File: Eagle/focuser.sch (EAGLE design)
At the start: 14 parts, among them IC1 L293D, IC2 L293D, IC3 PCF8574P

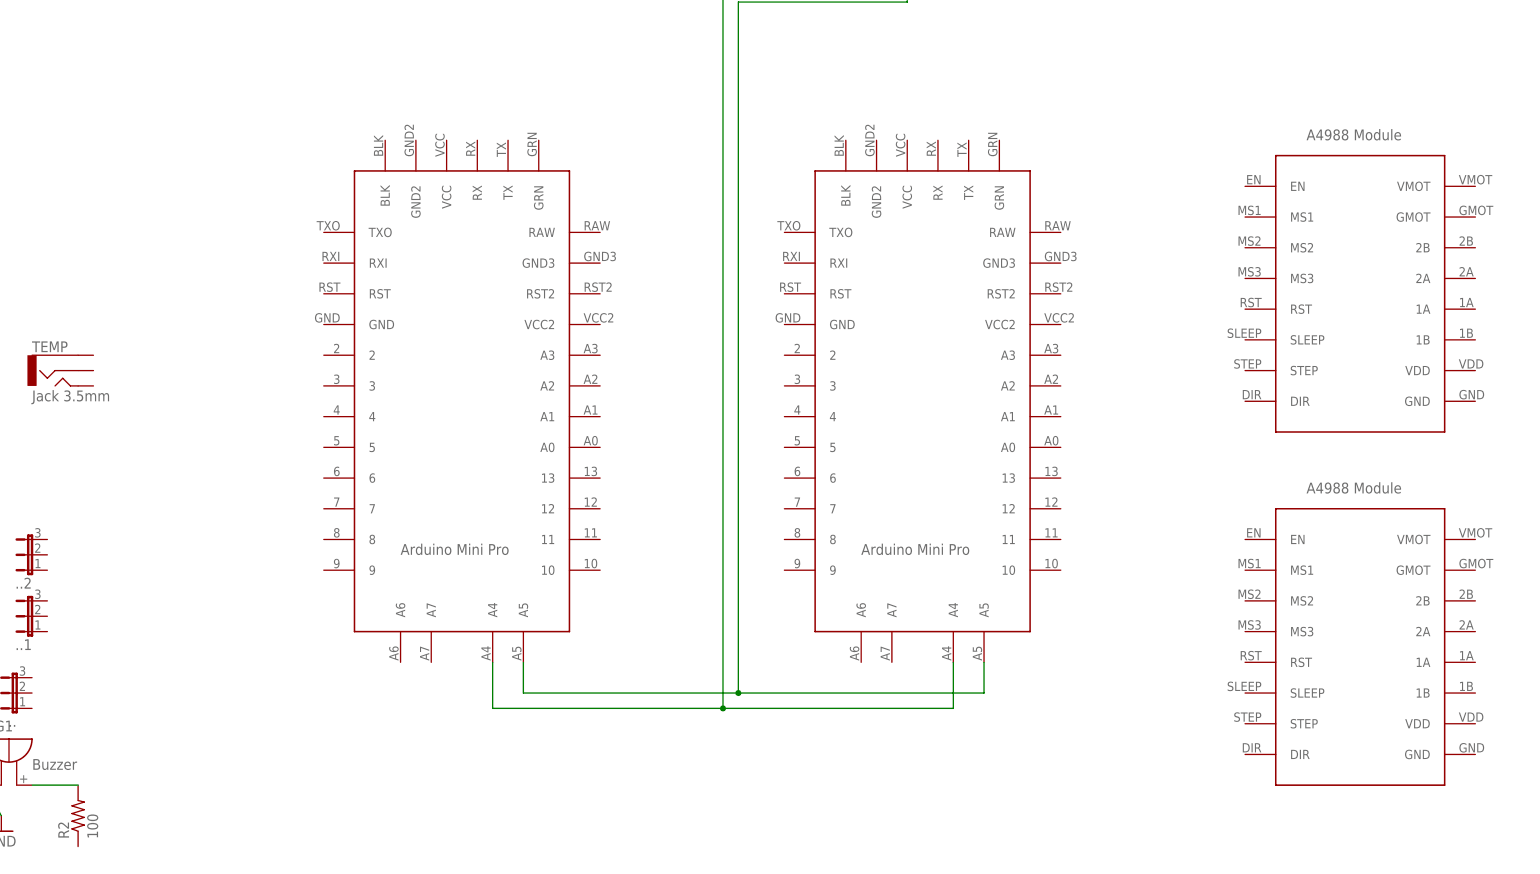
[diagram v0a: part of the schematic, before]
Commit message: Work continues... VB script update
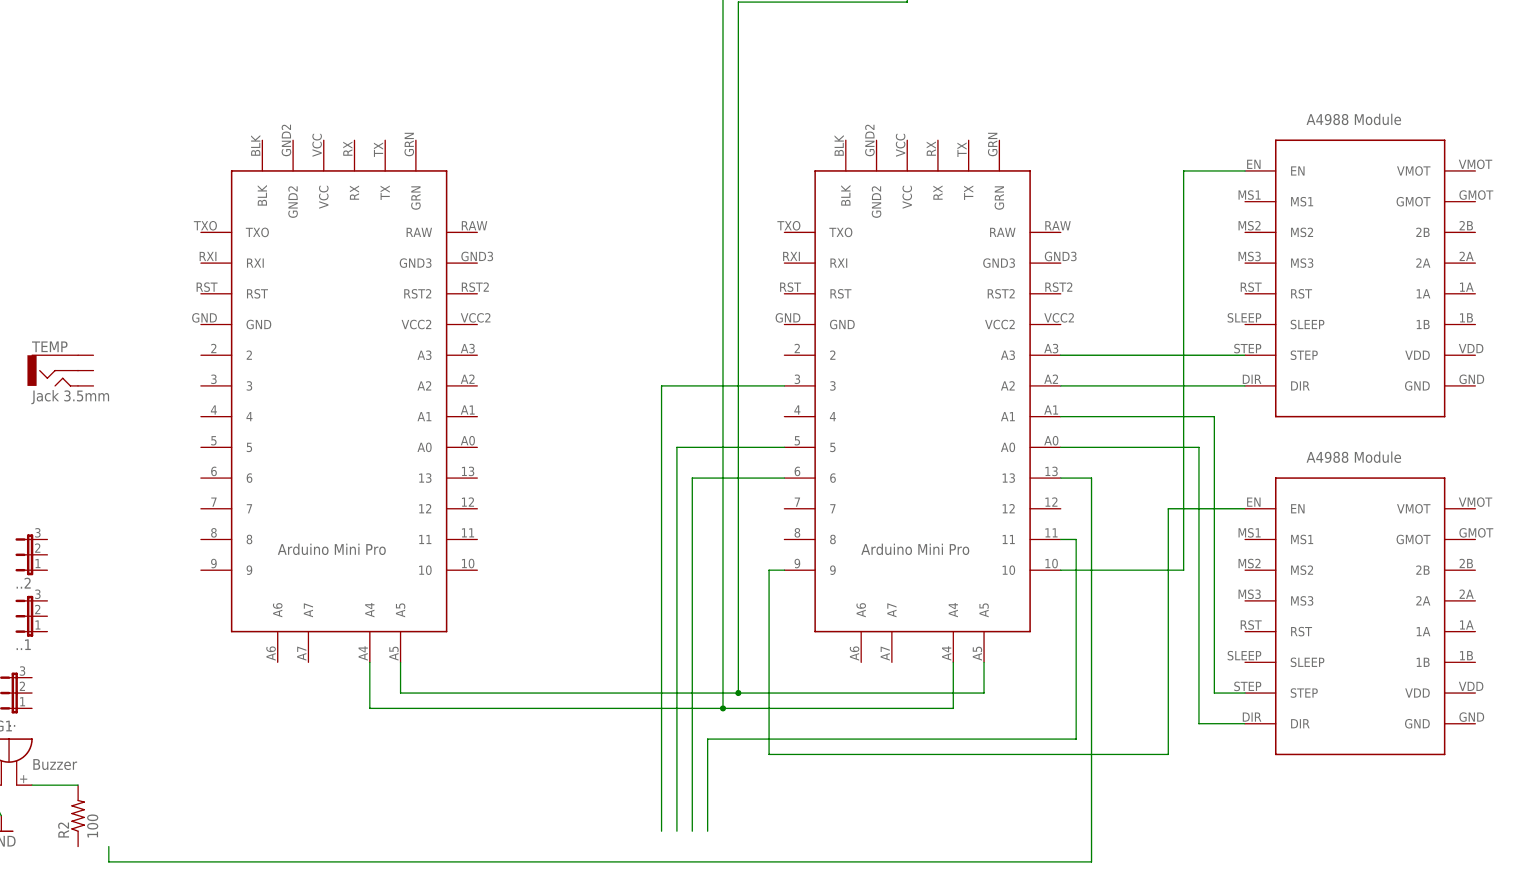
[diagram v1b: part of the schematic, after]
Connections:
- new net N$10: U$1.6
- new net N$11: U$1.5
- new net N$12: U$1.3
- new net N$13: U$1.11
- new net N$14: U$1.13
- new net N$3: U$1.A3, U$7.STEP
- new net N$4: U$1.A2, U$7.DIR
- new net N$5: U$1.A1, U$6.STEP
- new net N$6: U$1.A0, U$6.DIR
- new net N$7: U$1.10, U$7.EN
- new net N$8: U$1.9, U$6.EN
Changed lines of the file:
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@@
 <instance part="..2" gate="G$1" x="-33.02" y="45.72" rot="R90"/>
 <instance part="U$1" gate="G$1" x="116.84" y="81.28"/>
-<instance part="U$6" gate="G$1" x="182.88" y="38.1"/>
-<instance part="U$7" gate="G$1" x="182.88" y="96.52"/>
-<instance part="U$8" gate="G$1" x="40.64" y="81.28"/>
+<instance part="U$6" gate="G$1" x="182.88" y="43.18"/>
+<instance part="U$7" gate="G$1" x="182.88" y="99.06"/>
+<instance part="U$8" gate="G$1" x="20.32" y="81.28"/>
 <instance part="IC1" gate="G$1" x="190.5" y="160.02" rot="R90"/>
 <instance part="IC2" gate="G$1" x="190.5" y="210.82" rot="R90"/>
@@
 <net name="N$1" class="0">
 <segment>
-<pinref part="U$8" gate="G$1" pin="A5"/>
-<wire x1="48.26" y1="30.48" x2="48.26" y2="25.4" width="0.1524" layer="91"/>
-<wire x1="48.26" y1="25.4" x2="83.82" y2="25.4" width="0.1524" layer="91"/>
+<wire x1="27.94" y1="25.4" x2="83.82" y2="25.4" width="0.1524" layer="91"/>
 <pinref part="U$1" gate="G$1" pin="A5"/>
 <wire x1="83.82" y1="25.4" x2="124.46" y2="25.4" width="0.1524" layer="91"/>
@@
 <wire x1="83.82" y1="139.7" x2="83.82" y2="25.4" width="0.1524" layer="91"/>
 <junction x="83.82" y="25.4"/>
+<pinref part="U$8" gate="G$1" pin="A5"/>
+<wire x1="27.94" y1="30.48" x2="27.94" y2="25.4" width="0.1524" layer="91"/>
 </segment>
 </net>
 <net name="N$2" class="0">
 <segment>
-<pinref part="U$8" gate="G$1" pin="A4"/>
-<wire x1="43.18" y1="30.48" x2="43.18" y2="22.86" width="0.1524" layer="91"/>
-<wire x1="43.18" y1="22.86" x2="81.28" y2="22.86" width="0.1524" layer="91"/>
+<wire x1="22.86" y1="22.86" x2="81.28" y2="22.86" width="0.1524" layer="91"/>
 <pinref part="U$1" gate="G$1" pin="A4"/>
 <wire x1="81.28" y1="22.86" x2="119.38" y2="22.86" width="0.1524" layer="91"/>
@@
 <wire x1="81.28" y1="142.24" x2="81.28" y2="22.86" width="0.1524" layer="91"/>
 <junction x="81.28" y="22.86"/>
+<pinref part="U$8" gate="G$1" pin="A4"/>
+<wire x1="22.86" y1="22.86" x2="22.86" y2="30.48" width="0.1524" layer="91"/>
 </segment>
 </net>
+<net name="N$3" class="0">
+<segment>
+<pinref part="U$1" gate="G$1" pin="A3"/>
+<pinref part="U$7" gate="G$1" pin="STEP"/>
+<wire x1="137.16" y1="81.28" x2="167.64" y2="81.28" width="0.1524" layer="91"/>
+</segment>
+</net>
+<net name="N$4" class="0">
+<segment>
+<pinref part="U$1" gate="G$1" pin="A2"/>
+<pinref part="U$7" gate="G$1" pin="DIR"/>
+<wire x1="137.16" y1="76.2" x2="167.64" y2="76.2" width="0.1524" layer="91"/>
+</segment>
+</net>
+<net name="N$5" class="0">
+<segment>
+<pinref part="U$1" gate="G$1" pin="A1"/>
+<wire x1="137.16" y1="71.12" x2="162.56" y2="71.12" width="0.1524" layer="91"/>
+<wire x1="162.56" y1="71.12" x2="162.56" y2="25.4" width="0.1524" layer="91"/>
+<pinref part="U$6" gate="G$1" pin="STEP"/>
+<wire x1="162.56" y1="25.4" x2="167.64" y2="25.4" width="0.1524" layer="91"/>
+</segment>
+</net>
+<net name="N$6" class="0">
+<segment>
+<pinref part="U$1" gate="G$1" pin="A0"/>
+<wire x1="137.16" y1="66.04" x2="160.02" y2="66.04" width="0.1524" layer="91"/>
+<wire x1="160.02" y1="66.04" x2="160.02" y2="20.32" width="0.1524" layer="91"/>
+<pinref part="U$6" gate="G$1" pin="DIR"/>
+<wire x1="160.02" y1="20.32" x2="167.64" y2="20.32" width="0.1524" layer="91"/>
+</segment>
+</net>
+<net name="N$7" class="0">
+<segment>
+<pinref part="U$1" gate="G$1" pin="10"/>
+<wire x1="137.16" y1="45.72" x2="157.48" y2="45.72" width="0.1524" layer="91"/>
+<wire x1="157.48" y1="45.72" x2="157.48" y2="111.76" width="0.1524" layer="91"/>
+<pinref part="U$7" gate="G$1" pin="EN"/>
+<wire x1="157.48" y1="111.76" x2="167.64" y2="111.76" width="0.1524" layer="91"/>
+</segment>
+</net>
+<net name="N$8" class="0">
+<segment>
+<pinref part="U$1" gate="G$1" pin="9"/>
+<wire x1="91.44" y1="45.72" x2="88.9" y2="45.72" width="0.1524" layer="91"/>
+<wire x1="88.9" y1="45.72" x2="88.9" y2="15.24" width="0.1524" layer="91"/>
+<wire x1="88.9" y1="15.24" x2="154.94" y2="15.24" width="0.1524" layer="91"/>
+<wire x1="154.94" y1="15.24" x2="154.94" y2="55.88" width="0.1524" layer="91"/>
+<pinref part="U$6" gate="G$1" pin="EN"/>
+<wire x1="154.94" y1="55.88" x2="167.64" y2="55.88" width="0.1524" layer="91"/>
+</segment>
+</net>
+<net name="N$10" class="0">
+<segment>
+<pinref part="U$1" gate="G$1" pin="6"/>
+<wire x1="91.44" y1="60.96" x2="76.2" y2="60.96" width="0.1524" layer="91"/>
+<wire x1="76.2" y1="60.96" x2="76.2" y2="2.54" width="0.1524" layer="91"/>
+</segment>
+</net>
+<net name="N$11" class="0">
+<segment>
+<pinref part="U$1" gate="G$1" pin="5"/>
+<wire x1="91.44" y1="66.04" x2="73.66" y2="66.04" width="0.1524" layer="91"/>
+<wire x1="73.66" y1="66.04" x2="73.66" y2="2.54" width="0.1524" layer="91"/>
+</segment>
+</net>
+<net name="N$12" class="0">
+<segment>
+<pinref part="U$1" gate="G$1" pin="3"/>
+<wire x1="91.44" y1="76.2" x2="71.12" y2="76.2" width="0.1524" layer="91"/>
+<wire x1="71.12" y1="76.2" x2="71.12" y2="2.54" width="0.1524" layer="91"/>
+</segment>
+</net>
+<net name="N$13" class="0">
+<segment>
+<pinref part="U$1" gate="G$1" pin="11"/>
+<wire x1="137.16" y1="50.8" x2="139.7" y2="50.8" width="0.1524" layer="91"/>
+<wire x1="139.7" y1="50.8" x2="139.7" y2="17.78" width="0.1524" layer="91"/>
+<wire x1="139.7" y1="17.78" x2="78.74" y2="17.78" width="0.1524" layer="91"/>
+<wire x1="78.74" y1="17.78" x2="78.74" y2="2.54" width="0.1524" layer="91"/>
+</segment>
+</net>
+<net name="N$14" class="0">
+<segment>
+<pinref part="U$1" gate="G$1" pin="13"/>
+<wire x1="137.16" y1="60.96" x2="142.24" y2="60.96" width="0.1524" layer="91"/>
+<wire x1="142.24" y1="60.96" x2="142.24" y2="-2.54" width="0.1524" layer="91"/>
+<wire x1="142.24" y1="-2.54" x2="-20.32" y2="-2.54" width="0.1524" layer="91"/>
+<wire x1="-20.32" y1="-2.54" x2="-20.32" y2="0" width="0.1524" layer="91"/>
+</segment>
+</net>

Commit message: Schematic update
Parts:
- removed .., ..1, ..2: JUMPER-3PTH, SparkFun:JUMPER-3PTH
- removed IC3: PCF8574P, micro-philips:PCF8574P
- added 12V1, 12V2, 12V3, 12V4, 12V5, 12V6: Jack 5.5/2.1, SparkFun:POWER_JACKCOMBO
- added C1: 1000u, SparkFun:CAP_POLPTH4
- added C10, C8: 10u, SparkFun:CAP_POLPTH2
- added C2, C3, C4, C5, C6, C7, C9: 100n, SparkFun:CAPPTH1
- added D1, D2: (no value), SparkFun:DIODE1N4148
- added F1, F2, F3, F4, F5, F6, F7: PTCPTH, SparkFun:PTCPTH
- added IC4: L293D, st-microelectronics:L293D
- added IC5: 7809, SparkFun:V_REG_78XXSINK
- added IC6: ULN2003AN, uln-udn:ULN2003AN
- added J1, J2, J3, J4: POWER_JACKRCA, SparkFun:POWER_JACKRCA
- added Q1, Q2, Q3, Q4: IRF540, transistor-fet:IRF540
- added R1, R7, R8, R9: 100, SparkFun:RESISTORPTH1
- added R10, R11, R12, R3, R4, R5, R6: 3k3, SparkFun:RESISTORPTH1
- added TEMP1, TEMP2: Jack 3.5mm, SparkFun:AUDIO-JACKPTH
- added U$10, U$14: DCDC-5V, jolo-lib:DCDC-STEPDOWN
- added U$11, U$12, U$13, U$15, U$9: RELAYPTH, SparkFun:RELAYPTH
- added U$16: I2C, SparkFun:RJ9PTH
- added X1, X2: (no value), SparkFun:DB9
- IC2: MPN (none) -> L293D; OC_FARNELL (none) -> 9589619; OC_NEWARK (none) -> 56P8249
- U$6: value A4988-MODULE -> SW motor; device jolo-lib:A4988-MODULE -> SparkFun:RJ9PTH
- U$7: value A4988-MODULE -> Hand control; device jolo-lib:A4988-MODULE -> SparkFun:RJ9PTH
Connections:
- removed net GND: SG1.+
- new net +12V: 12V.PWR, 12V5.PWR, C1.+, C2.1, C3.1, C9.1, F1.1, F2.1, F3.2, IC5.IN, IC6.CD+, J1.PWR, J2.PWR, J3.PWR, J4.PWR, U$11.COIL2, U$11.MAIN, U$12.COIL2, U$12.MAIN, U$13.COIL2, U$13.MAIN, U$15.COIL2, U$9.COIL2, U$9.MAIN
- new net +5V: C10.+, C4.2, C5.2, C8.+, IC1.VCC2, IC2.VCC2, IC4.VCC2, R10.2, R11.2, R12.2, TEMP.5, TEMP1.5, TEMP2.5, U$1.VCC2, U$10.VCCOUT, U$16.4, U$7.4, U$8.VCC2
- new net 3.3V: C7.1, IC4.VCC1, IC5.OUT
- new net AGND: 12V.GND, 12V.GNDBREAK, 12V1.GND, 12V1.GNDBREAK, 12V2.GND, 12V2.GNDBREAK, 12V3.GND, 12V3.GNDBREAK, 12V4.GND, 12V4.GNDBREAK, 12V5.GND, 12V5.GNDBREAK, 12V6.GND, 12V6.GNDBREAK, C1.-, C2.2, C3.2, C6.2, C7.2, C9.2, IC1.GND1, IC1.GND2, IC1.GND3, IC1.GND4, IC2.GND1, IC2.GND2, IC2.GND3, IC2.GND4, IC4.GND1, IC4.GND2, IC4.GND3, IC4.GND4, IC5.GND, Q1.S, Q2.S, Q3.S, Q4.S, R3.2, R4.2, R5.2, R6.2, X1.9, X2.9
- new net DGND: C10.-, C4.1, C5.1, C8.-, SG1.+, TEMP.1, TEMP1.1, TEMP2.1, U$1.GND, U$10.GNDIN, U$10.GNDOUT, U$14.GNDIN, U$14.GNDOUT, U$16.1, U$7.1, U$8.GND
- new net N$15: IC2.2Y, X2.1
- new net N$16: IC1.2Y, X1.1
- new net N$17: D1.C, D2.C, R2.1
- new net N$18: IC6.I1, U$8.8
- new net N$19: IC1.2A, U$1.2
- new net N$20: IC1.1A, U$1.4
- new net N$21: IC2.3A, U$1.8
- new net N$22: IC2.4A, U$1.7
- new net N$23: IC6.I2, U$8.7
- new net N$25: IC6.I3, U$8.6
- new net N$27: IC6.I4, U$8.5
- new net N$28: U$7.2, U$8.A0
- new net N$30: IC4.1-2EN, IC4.3-4EN, U$8.9
- new net N$35: J1.GND, J1.GNDBREAK, Q1.D
- new net N$36: J2.GND, J2.GNDBREAK, Q2.D
- new net N$37: 12V6.PWR, U$15.NO
- new net N$38: J3.GND, J3.GNDBREAK, Q3.D
- new net N$39: Q4.G, R6.1, R9.1
- new net N$40: Q3.G, R5.1, R8.1
- new net N$41: Q2.G, R4.1, R7.1
- new net N$42: Q1.G, R1.1, R3.1
- new net N$43: 12V1.PWR, F4.1
- new net N$45: IC4.3Y, U$6.4
- new net N$46: D1.A, U$8.13
- new net N$47: R9.2, U$1.11
- new net N$48: R8.2, U$1.3
- new net N$49: R7.2, U$1.5
- new net N$50: R1.2, U$1.6
- new net N$51: U$6.3
- new net N$52: 12V2.PWR, F5.1
- new net N$54: IC6.O5, U$9.COIL1
- new net N$55: IC6.O4, U$11.COIL1
- new net N$56: IC6.O3, U$12.COIL1
- new net N$57: IC6.O2, U$13.COIL1
- new net N$58: C6.1, F3.1, IC1.VCC1, IC2.VCC1, X1.5, X2.5
- new net N$59: R12.1, TEMP.2, U$8.A1
- new net N$60: 12V3.PWR, F6.1
- new net N$61: 12V4.PWR, F7.1
- new net N$62: F7.2, U$13.NO
- new net N$63: IC6.O1, U$15.COIL1
- new net N$64: J4.GND, J4.GNDBREAK, Q4.D
- new net N$65: R11.1, TEMP1.2, U$8.A2
- new net N$66: F6.2, U$12.NO
- new net N$67: F5.2, U$11.NO
- new net N$68: F4.2, U$9.NO
- new net N$69: F1.2, U$10.VCCIN
- new net N$70: F2.2, U$14.VCCIN
- new net N$71: R10.1, TEMP2.2, U$8.A3
- new net N$73: IC2.3Y, X2.4
- new net N$74: IC4.4A, U$8.11
- new net N$75: IC4.3A, U$8.10
- new net N$9: IC1.4A, U$1.A2
- new net V+: U$14.VCCOUT, U$15.MAIN
- net N$1: now also U$16.2; no longer IC3.SCL
- net N$10: now also IC2.1A, U$1.A1; no longer U$1.6
- net N$11: now also IC2.2A, U$1.A0; no longer U$1.5
- net N$12: now also IC2.1-2EN, IC2.3-4EN, U$1.10; no longer U$1.3
- net N$13: now also IC2.1Y, X2.2; no longer U$1.11
- net N$14: now also D2.A
- net N$2: now also U$16.3; no longer IC3.SDA
- net N$3: now also IC1.3A; no longer U$7.STEP
- net N$4: now also IC2.4Y, X2.3; no longer U$1.A2, U$7.DIR
- net N$5: now also IC1.1Y, X1.2; no longer U$1.A1, U$6.STEP
- net N$6: now also IC1.4Y, X1.3; no longer U$1.A0, U$6.DIR
- net N$7: now also IC1.3Y, X1.4; no longer U$1.10, U$7.EN
- net N$8: now also IC1.3-4EN; no longer U$6.EN
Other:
- moved on the sheet: 12V, IC1, IC2, R2, SG1, TEMP
